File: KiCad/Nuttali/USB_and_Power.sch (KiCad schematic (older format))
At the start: 14 parts, among them J2 B4B-XH-A, U3 USBLC6-2P6, U4 AP131-15, U5 AP1117-15

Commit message: extended the pcb board with 2 mm to right
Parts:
- C22, C23, C24, C25, C26: symbol Device:C -> Nuttali-rescue:C-Device
- D1, D2: symbol Device:LED -> Nuttali-rescue:LED-Device
- R4, R5, R6: symbol Device:R -> Nuttali-rescue:R-Device
- U3: symbol Power_Protection:USBLC6-2P6 -> Nuttali-rescue:USBLC6-2P6-Power_Protection
- U4: symbol Regulator_Linear:AP131-15 -> Nuttali-rescue:AP131-15-Regulator_Linear
- U5: symbol Regulator_Linear:AP1117-15 -> Nuttali-rescue:AP1117-15-Regulator_Linear
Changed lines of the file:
@@
 $EndComp
 $Comp
-L power:+5V #PWR0126
+L Nuttali-rescue:+5V-power #PWR0126
 U 1 1 6025442C
 P 1850 1500
@@
 	1850 1600 1850 1500
 $Comp
-L Power_Protection:USBLC6-2P6 U3
+L Nuttali-rescue:USBLC6-2P6-Power_Protection U3
 U 1 1 60257671
 P 3450 1800
@@
 	3350 2250 3350 2200
 $Comp
-L power:+5V #PWR0127
+L Nuttali-rescue:+5V-power #PWR0127
 U 1 1 60263555
 P 2350 1600
@@
 	1600 1900 1850 1900
 $Comp
-L power:GND #PWR0128
+L Nuttali-rescue:GND-power #PWR0128
 U 1 1 60263C21
 P 1850 1900
@@
 	3850 1800 3900 1800
 $Comp
-L power:GND #PWR0129
+L Nuttali-rescue:GND-power #PWR0129
 U 1 1 6026528C
 P 3900 1800
@@
 	3550 2250 3550 2200
 $Comp
-L Regulator_Linear:AP1117-15 U5
+L Nuttali-rescue:AP1117-15-Regulator_Linear U5
 U 1 1 60275CC9
 P 5150 1550
@@
 $EndComp
 $Comp
-L Device:C C22
+L Nuttali-rescue:C-Device C22
 U 1 1 601D7AEF
 P 2350 1950
@@
 	2800 2000 2950 2000
 $Comp
-L power:GND #PWR0130
+L Nuttali-rescue:GND-power #PWR0130
 U 1 1 601DAD67
 P 2950 2000
@@
 $EndComp
 $Comp
-L Device:C C25
+L Nuttali-rescue:C-Device C25
 U 1 1 601DF5EF
 P 5700 1800
@@
 $EndComp
 $Comp
-L Device:C C24
+L Nuttali-rescue:C-Device C24
 U 1 1 601E048D
 P 4600 2950
@@
 $EndComp
 $Comp
-L Device:C C26
+L Nuttali-rescue:C-Device C26
 U 1 1 601E088B
 P 5950 2800
@@
 	5150 2000 5700 2000
 $Comp
-L power:GND #PWR0131
+L Nuttali-rescue:GND-power #PWR0131
 U 1 1 601E6056
 P 5150 2000
@@
 $EndComp
 $Comp
-L Device:R R4
+L Nuttali-rescue:R-Device R4
 U 1 1 601E6FBD
 P 5600 2800
@@
 $EndComp
 $Comp
-L Device:R R5
+L Nuttali-rescue:R-Device R5
 U 1 1 601E7C9F
 P 5600 3200
@@
 	5050 3350 5600 3350
 $Comp
-L power:GND #PWR0132
+L Nuttali-rescue:GND-power #PWR0132
 U 1 1 601F167A
 P 5050 3350
@@
 $EndComp
 $Comp
-L power:+5V #PWR0133
+L Nuttali-rescue:+5V-power #PWR0133
 U 1 1 601F267E
 P 4600 1500
@@
 $EndComp
 $Comp
-L power:+5V #PWR0134
+L Nuttali-rescue:+5V-power #PWR0134
 U 1 1 601F2F4A
 P 4600 2600
@@
 	5950 2950 5950 3000
 $Comp
-L power:GND #PWR0135
+L Nuttali-rescue:GND-power #PWR0135
 U 1 1 601F601B
 P 5950 3000
@@
 $EndComp
 $Comp
-L power:+3.3V #PWR0137
+L Nuttali-rescue:+3.3V-power #PWR0137
 U 1 1 601F8551
 P 5700 1500
@@
 $EndComp
 $Comp
-L Device:LED D1
+L Nuttali-rescue:LED-Device D1
 U 1 1 60219D13
 P 6250 2650
@@
 	6400 2650 6500 2650
 $Comp
-L power:GND #PWR0138
+L Nuttali-rescue:GND-power #PWR0138
 U 1 1 6021DE9A
 P 6500 2650
@@
 	5700 1550 5700 1650
 $Comp
-L Device:R R6
+L Nuttali-rescue:R-Device R6
 U 1 1 60221CF5
 P 6200 1550
@@
 $EndComp
 $Comp
-L Device:LED D2
+L Nuttali-rescue:LED-Device D2
 U 1 1 60223427
 P 6550 1550
@@
 	6700 1550 6700 1600
 $Comp
-L power:GND #PWR0139
+L Nuttali-rescue:GND-power #PWR0139
 U 1 1 60225F08
 P 6700 1600
@@
 	5700 2000 5700 1950
 $Comp
-L Device:C C23
+L Nuttali-rescue:C-Device C23
 U 1 1 6022CD87
 P 4600 1800
@@
 	5050 3050 5050 3350
 $Comp
-L Regulator_Linear:AP131-15 U4
+L Nuttali-rescue:AP131-15-Regulator_Linear U4
 U 1 1 602779E7
 P 5050 2750

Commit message: Fixed almost all footprints and nearly the layout of the pcb
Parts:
- D1, D2: footprint LED_SMD:LED_0201_0603Metric_Pad0.64x0.40mm_HandSolder -> Nuttali:LED
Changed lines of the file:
@@
 F 0 "D1" H 6243 2395 50  0000 C CNN
 F 1 "LED" H 6243 2486 50  0000 C CNN
-F 2 "LED_SMD:LED_0201_0603Metric_Pad0.64x0.40mm_HandSolder" H 6250 2650 50  0001 C CNN
+F 2 "Nuttali:LED" H 6250 2650 50  0001 C CNN
 F 3 "~" H 6250 2650 50  0001 C CNN
 	1    6250 2650
@@
 F 0 "D2" H 6543 1295 50  0000 C CNN
 F 1 "LED" H 6543 1386 50  0000 C CNN
-F 2 "LED_SMD:LED_0201_0603Metric_Pad0.64x0.40mm_HandSolder" H 6550 1550 50  0001 C CNN
+F 2 "Nuttali:LED" H 6550 1550 50  0001 C CNN
 F 3 "~" H 6550 1550 50  0001 C CNN
 	1    6550 1550

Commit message: Finnished the pcb
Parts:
- U5: footprint Package_TO_SOT_SMD:SOT-223-3_TabPin2 -> Package_TO_SOT_SMD:SOT-23
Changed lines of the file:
@@
 F 0 "U5" H 5150 1792 50  0000 C CNN
 F 1 "AP1117-15" H 5150 1701 50  0000 C CNN
-F 2 "Package_TO_SOT_SMD:SOT-223-3_TabPin2" H 5150 1750 50  0001 C CNN
+F 2 "Package_TO_SOT_SMD:SOT-23" H 5150 1750 50  0001 C CNN
 F 3 "http://www.diodes.com/datasheets/AP1117.pdf" H 5250 1300 50  0001 C CNN
 	1    5150 1550

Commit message: PCB done
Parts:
- U3: footprint Package_TO_SOT_SMD:SOT-666 -> PMW:SOT-666_ESD
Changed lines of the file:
@@
 F 0 "U3" V 3100 2400 50  0000 C CNN
 F 1 "USBLC6-2P6" V 3200 2400 50  0000 C CNN
-F 2 "Package_TO_SOT_SMD:SOT-666" H 3450 1300 50  0001 C CNN
+F 2 "PMW:SOT-666_ESD" H 3450 1300 50  0001 C CNN
 F 3 "https://www.st.com/resource/en/datasheet/usblc6-2.pdf" H 3650 2150 50  0001 C CNN
 	1    3450 1800

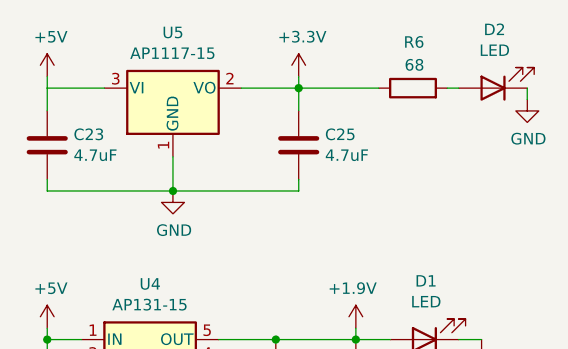
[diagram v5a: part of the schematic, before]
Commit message: added pers things to project
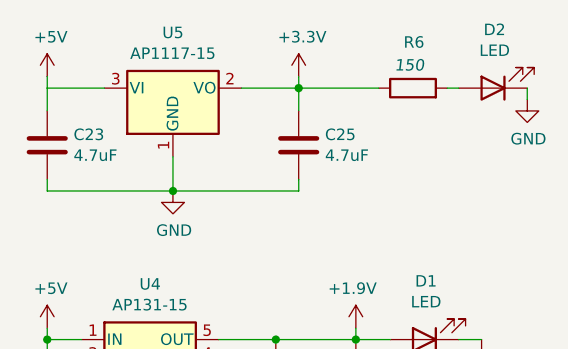
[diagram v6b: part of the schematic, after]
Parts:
- R6: value 68 -> 150
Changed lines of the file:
@@
 P 6200 1550
 F 0 "R6" V 6400 1500 50  0000 L CNN
-F 1 "68" V 6300 1500 50  0000 L CNN
+F 1 "150" V 6300 1500 50  0000 L CIN
 F 2 "Resistor_SMD:R_0805_2012Metric_Pad1.20x1.40mm_HandSolder" V 6130 1550 50  0001 C CNN
 F 3 "~" H 6200 1550 50  0001 C CNN
